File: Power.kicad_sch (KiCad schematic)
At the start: 22 parts, among them J3 Barrel_Jack_Switch, SW1 SW_Nidec_CAS-120A1, U3 TPS562202S, U4 TPS562202S

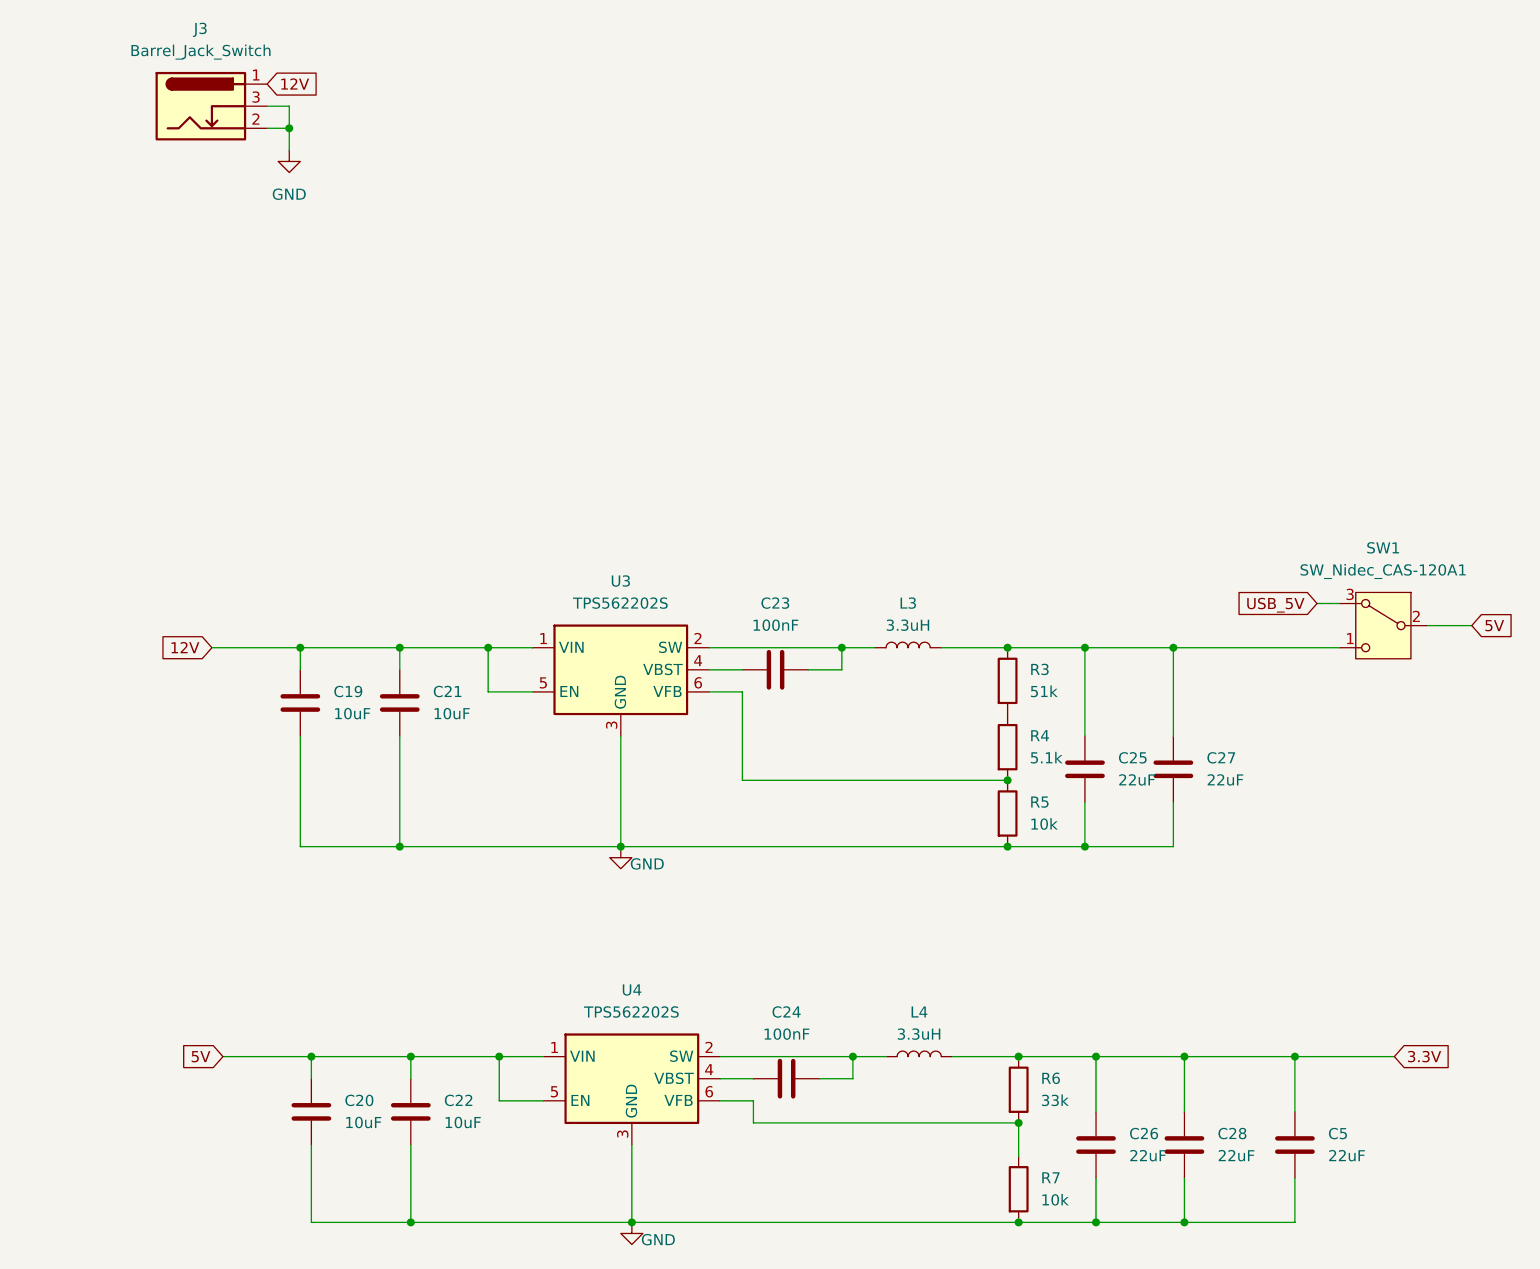
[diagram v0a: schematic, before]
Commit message: Add files via upload
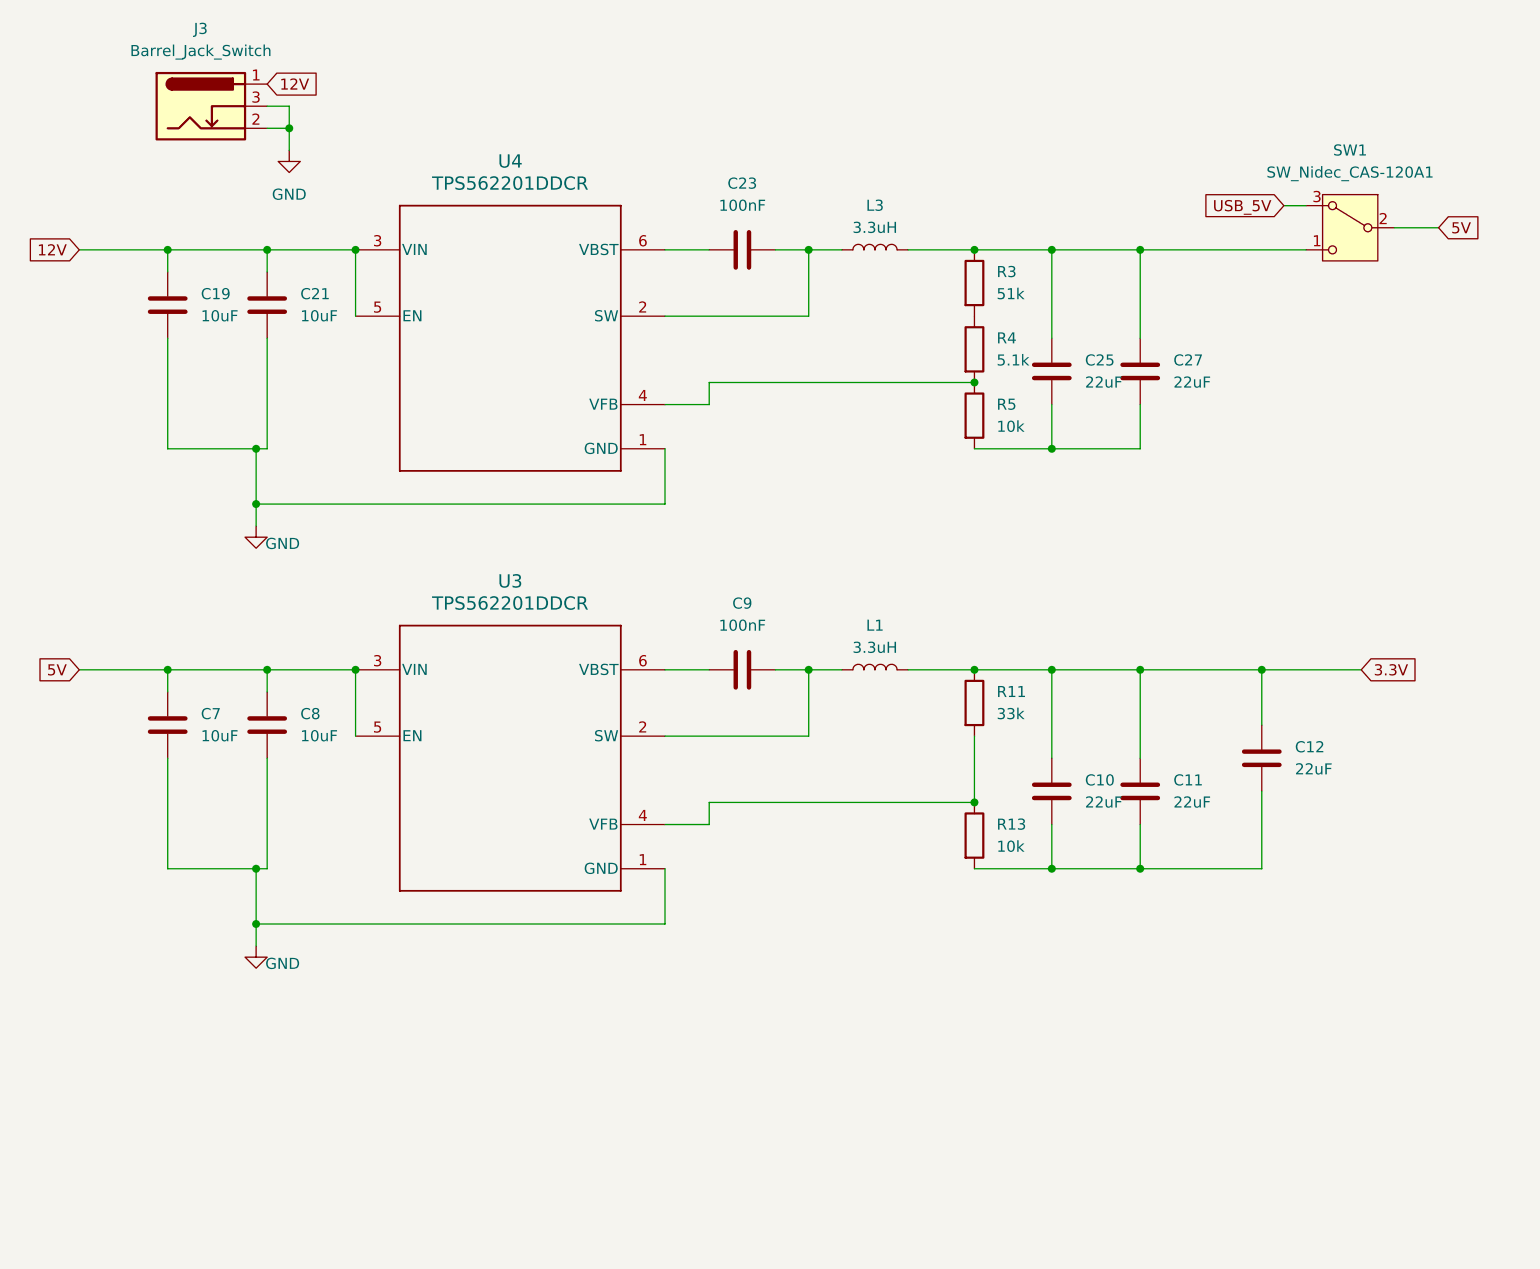
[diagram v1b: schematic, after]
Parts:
- removed C20, C22: 10uF, Capacitor_SMD:C_0805_2012Metric_Pad1.18x1.45mm_HandSolder, symbol Device:C
- removed C24: 100nF, Capacitor_SMD:C_0805_2012Metric_Pad1.18x1.45mm_HandSolder, symbol Device:C
- removed C26, C28, C5: 22uF, Capacitor_SMD:C_0805_2012Metric_Pad1.18x1.45mm_HandSolder, symbol Device:C
- removed L4: 3.3uH, Inductor_SMD:L_1008_2520Metric_Pad1.43x2.20mm_HandSolder, symbol Device:L
- removed R6: 33k, Resistor_SMD:R_0805_2012Metric_Pad1.20x1.40mm_HandSolder, symbol Device:R
- removed R7: 10k, Resistor_SMD:R_0805_2012Metric_Pad1.20x1.40mm_HandSolder, symbol Device:R
- removed U3, U4: TPS562202S, Package_TO_SOT_SMD:SOT-563, symbol Regulator_Switching:TPS562202S
- added C10, C11, C12: 22uF, Capacitor_SMD:C_0805_2012Metric_Pad1.18x1.45mm_HandSolder, symbol Device:C
- added C7, C8: 10uF, Capacitor_SMD:C_0805_2012Metric_Pad1.18x1.45mm_HandSolder, symbol Device:C
- added C9: 100nF, Capacitor_SMD:C_0805_2012Metric_Pad1.18x1.45mm_HandSolder, symbol Device:C
- added L1: 3.3uH, Inductor_SMD:L_1008_2520Metric_Pad1.43x2.20mm_HandSolder, symbol Device:L
- added R11: 33k, Resistor_SMD:R_0805_2012Metric_Pad1.20x1.40mm_HandSolder, symbol Device:R
- added R13: 10k, Resistor_SMD:R_0805_2012Metric_Pad1.20x1.40mm_HandSolder, symbol Device:R
- added U3, U4: TPS562201DDCR, Weather Station:DDC0006A_M, symbol regulator:TPS562201DDCR
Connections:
- net 12V: now also U4.3 (VIN), U4.5 (EN)
- net 3.3V: now also C10.1, C11.1, C12.1, L1.2, R11.1
- net 5V: now also C7.1, C8.1, U3.3 (VIN), U3.5 (EN)
- net GND: now also C7.2, C8.2, U3.1 (GND), U4.1 (GND); no longer C25.2, C27.2, R5.2
- net at C23.2, L3.1: now also U4.2 (SW)
- net at C23.1: now also U4.6 (VBST)
- net at R4.2, R5.1: now also U4.4 (VFB)
- new net: C10.2, C11.2, C12.2, R13.2
- new net: C25.2, C27.2, R5.2
- new net: C9.2, L1.1, U3.2 (SW)
- new net: C9.1, U3.6 (VBST)
- new net: R11.2, R13.1, U3.4 (VFB)
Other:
- moved on the sheet: C19, C21, C23, C25, C27, L3, R3, R4, R5, SW1
